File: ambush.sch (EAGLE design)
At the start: 159 parts, among them IC1 LM555N, IC10 LM555N, IC11 7430N, IC12 7400N, IC13 LM386N-3, IC14 74LS93N, IC15 74LS93N, IC16 7410N, IC17 7402N, IC18 7402N, IC19 7486N, IC2 7404N, IC20 74125N, IC21 7400N, IC22 LM555N, IC23 LM555N, IC24 7400N, IC25 LM555N, IC26 LM555N, IC27 74S20N, IC28 7404N, IC29 LM555N, IC3 LM555N, IC30 7400N, IC31 7475N, IC32 7485N, IC33 7485N, IC34 LM555N, IC35 LM555N, IC36 7402N, IC37 7404N, IC38 7400N, IC39 7404N, IC4 LM555N, IC40 7490N, IC41 7490N, IC42 4511N, IC43 4511N, IC44 74LS92N, IC45 7490N, IC46 7490N, IC47 7490N, IC48 4511N, IC49 4511N, IC5 7404N, IC50 7400N, IC6 74LS93N, IC7 LM555N, IC8 LM555N, IC9 74LS93N, T1 2N3904, T2 2N3904, T3 2N3904, T4 2N3904, T5 2N3904, T6 2N3904, Y1 14.3 MHz

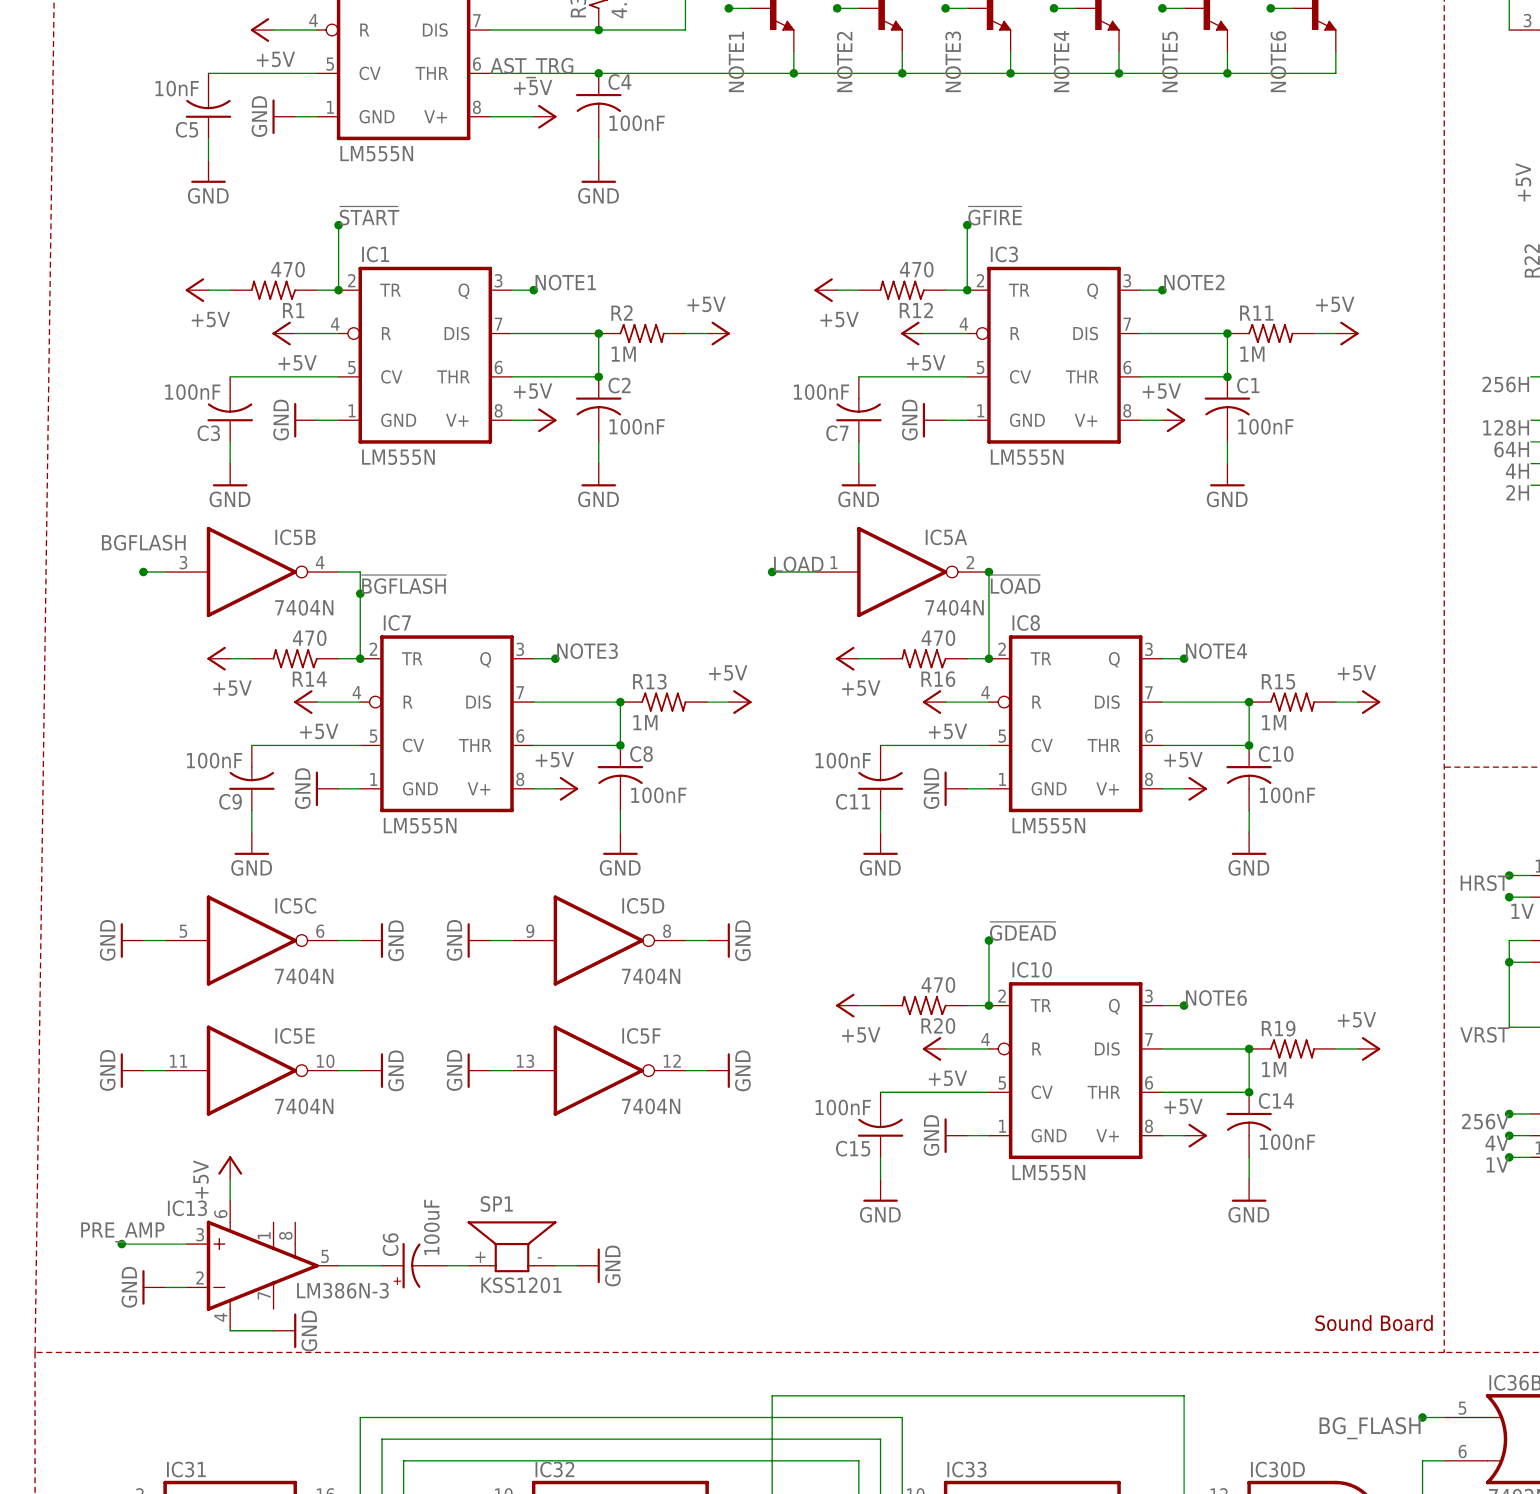
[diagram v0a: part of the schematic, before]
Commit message: -optimized the sound circuitry
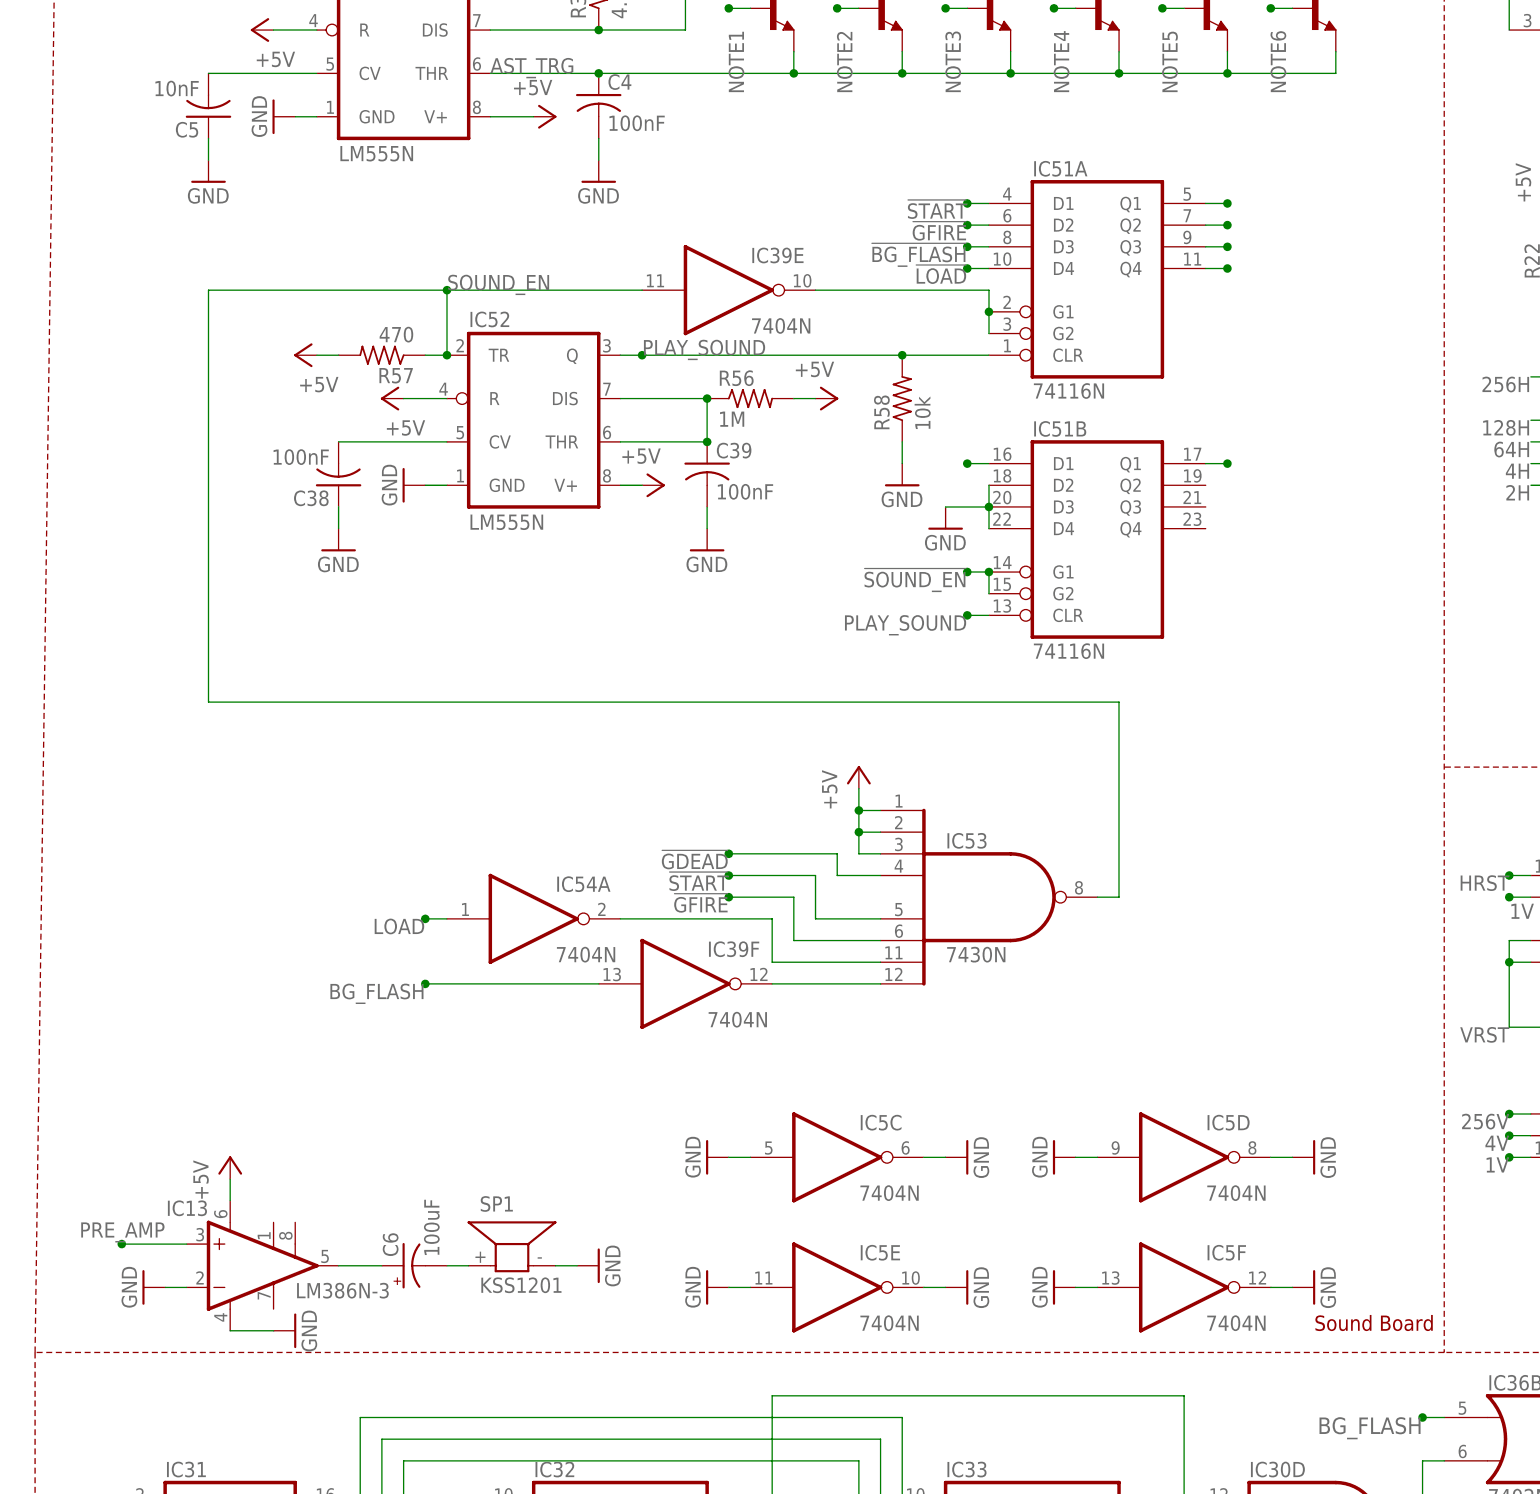
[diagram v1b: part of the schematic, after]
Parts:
- removed C1, C10, C11, C14, C15, C2, C3, C7, C8, C9: 100nF, resistor:C-US025-040X050
- removed IC1, IC10, IC3, IC7, IC8: LM555N, linear:LM555N
- removed R1, R12, R14, R16, R20: 470, resistor:R-US_0207/10
- removed R11, R13, R15, R19, R2: 1M, resistor:R-US_0207/10
- added C38, C39: 100nF, resistor:C-US025-040X050
- added IC51: 74116N, 74xx-us:74116N
- added IC52: LM555N, linear:LM555N
- added IC53: 7430N, 74xx-us:7430N
- added IC54: 7404N, 74xx-us:7404N
- added R56: 1M, resistor:R-US_0207/10
- added R57: 470, resistor:R-US_0207/10
- added R58: 10k, resistor:R-US_0207/10
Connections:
- removed net !BGFLASH: IC5B.O, IC7.TR, R14.1
- removed net BGFLASH: IC5B.I
- removed net N$1: C1.1, IC3.DIS, IC3.THR, R11.1
- removed net N$2: C7.2, IC3.CV
- removed net N$20: C14.1, IC10.DIS, IC10.THR, R19.1
- removed net N$22: C15.2, IC10.CV
- removed net N$3: C8.1, IC7.DIS, IC7.THR, R13.1
- removed net N$4: C9.2, IC7.CV
- removed net N$5: C2.1, IC1.DIS, IC1.THR, R2.1
- removed net N$6: C10.1, IC8.DIS, IC8.THR, R15.1
- removed net N$7: C3.2, IC1.CV
- removed net N$8: C11.2, IC8.CV
- new net !BG_FLASH: IC39F.O, IC51A.D3, IC53A.I7
- new net !SOUND_EN: IC39E.O, IC51A.G1, IC51A.G2, IC51B.G1, IC51B.G2
- new net N$128: C39.1, IC52.DIS, IC52.THR, R56.1
- new net N$152: C38.2, IC52.CV
- new net PLAY_SOUND: IC51A.CLR, IC51B.CLR, IC52.Q, R58.2
- new net SOUND_EN: IC39E.I, IC52.TR, IC53A.O, R57.1
- net !GDEAD: now also IC51B.D1, IC53A.I3; no longer IC10.TR, R20.1
- net !GFIRE: now also IC51A.D2, IC53A.I5; no longer IC3.TR, R12.1
- net !LOAD: now also IC51A.D4, IC53A.I6, IC54A.O; no longer IC5A.O, IC8.TR, R16.1
- net !START: now also IC51A.D1, IC53A.I4; no longer IC1.TR, R1.1
- net +5V: now also IC52.R, IC52.V+, IC53A.I0, IC53A.I1, IC53A.I2, R56.2, R57.2; no longer IC1.R, IC1.V+, IC10.R, IC10.V+, IC3.R, IC3.V+, IC7.R, IC7.V+, IC8.R, IC8.V+, R1.2, R11.2, R12.2, R13.2, R14.2, R15.2, R16.2, R19.2, R2.2, R20.2
- net BG_FLASH: now also IC39F.I
- net GND: now also C38.1, C39.2, IC51B.D2, IC51B.D3, IC51B.D4, IC52.GND, R58.1; no longer C1.2, C10.2, C11.1, C14.2, C15.1, C2.2, C3.1, C7.1, C8.2, C9.1, IC1.GND, IC10.GND, IC3.GND, IC7.GND, IC8.GND
- net LOAD: now also IC54A.I; no longer IC5A.I
- net NOTE1: now also IC51A.Q1; no longer IC1.Q
- net NOTE2: now also IC51A.Q2; no longer IC3.Q
- net NOTE3: now also IC51A.Q3; no longer IC7.Q
- net NOTE4: now also IC51A.Q4; no longer IC8.Q
- net NOTE5: now also IC51B.Q1
- net NOTE6: no longer IC10.Q
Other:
- moved on the sheet: IC5C, IC5D, IC5E, IC5F
